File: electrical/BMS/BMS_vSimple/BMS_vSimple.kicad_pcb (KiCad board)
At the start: 2 copper layers, 133.3 x 82.6 mm, 140 parts, among them J1 Conn_01x04_Pin, J2 Conn_02x12_Top_Bottom, J3 Conn_01x13_Socket, Q6 BCP56, U1 STM32F412RGTx, U2 BQ79652PAPRQ1, U3 ISO1044BD, U4 CD74HC4067M

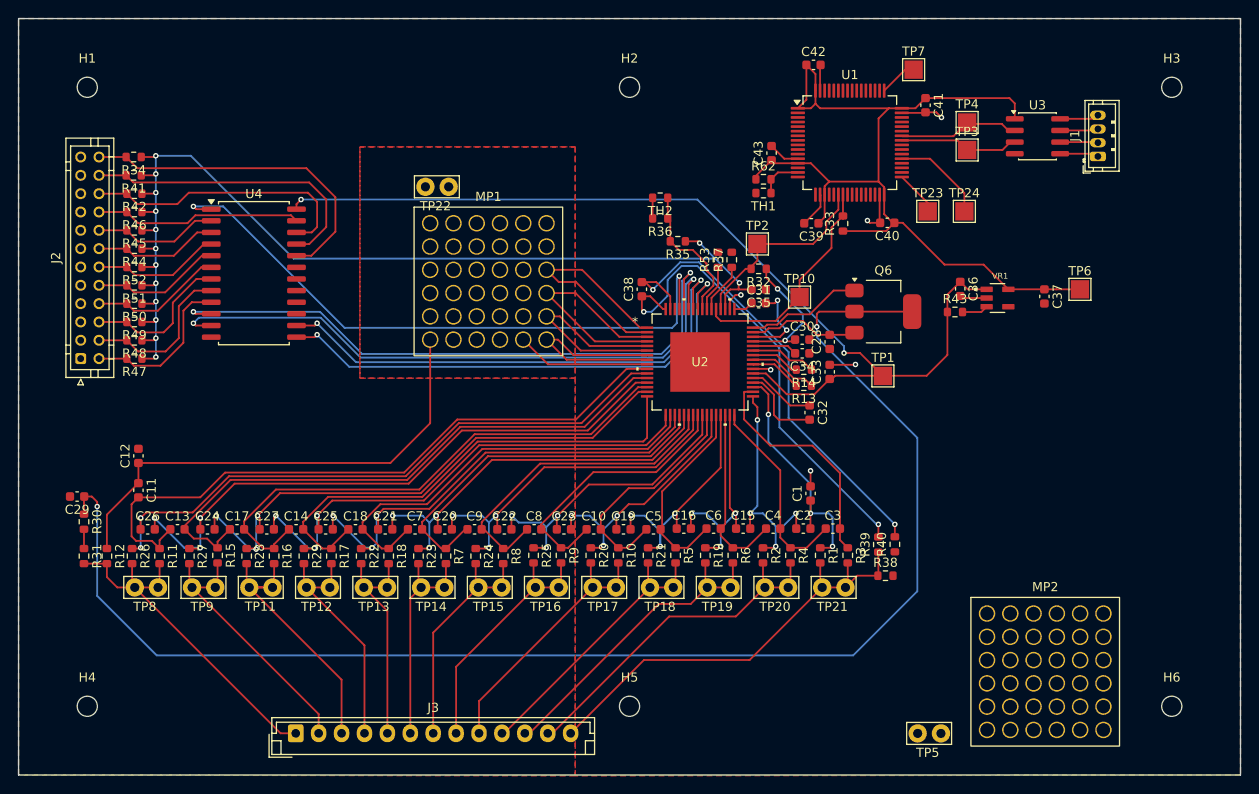
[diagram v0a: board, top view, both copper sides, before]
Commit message: bms is smaller now...
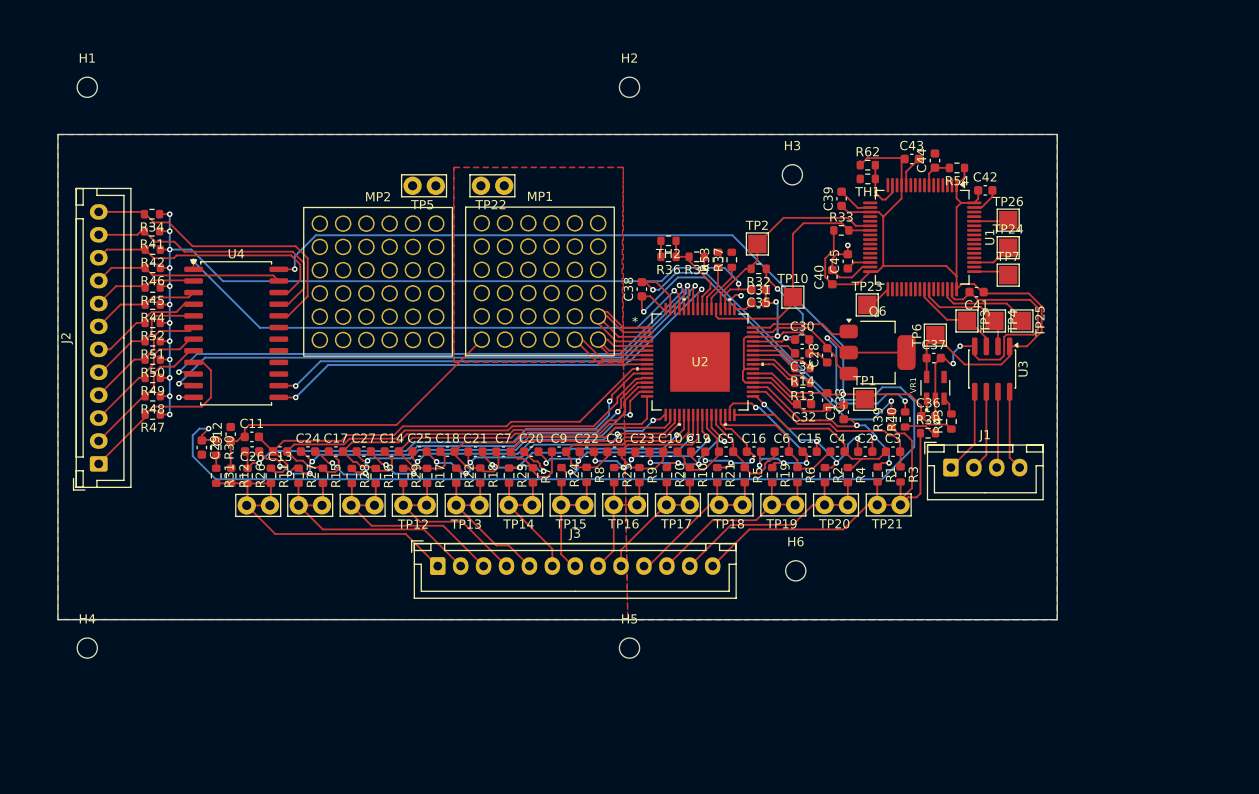
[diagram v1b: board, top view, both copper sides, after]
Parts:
- added C44: 100n, Capacitor_SMD:C_0603_1608Metric, F.Cu at (127.3, 75.8)
- added C45: 4.7u, Capacitor_SMD:C_0603_1608Metric, F.Cu at (117.8, 86.8)
- added R54: 10k, Resistor_SMD:R_0603_1608Metric, F.Cu at (129.7, 76.5)
- added TP25: TestPoint, TestPoint:TestPoint_Pad_2.0x2.0mm, F.Cu at (136.8, 93.2)
- added TP26: TestPoint, TestPoint:TestPoint_Pad_2.0x2.0mm, F.Cu at (135.2, 82.2)
- J1: footprint Connector_JST:JST_ZH_B4B-ZR_1x04_P1.50mm_Vertical -> Connector_JST:JST_XH_B4B-XH-A_1x04_P2.50mm_Vertical
- J2: value Conn_02x12_Top_Bottom -> Conn_01x12; footprint Connector_JST:JST_PHD_B24B-PHDSS_2x12_P2.00mm_Vertical -> Connector_JST:JST_XH_B12B-XH-A_1x12_P2.50mm_Vertical
- J3: footprint Connector_JST:JST_EH_B13B-EH-A_1x13_P2.50mm_Vertical -> Connector_JST:JST_XH_B13B-XH-A_1x13_P2.50mm_Vertical
- moved MP2 84.3 mm to (66.5, 89.0)
- moved TP5 81.3 mm to (70.2, 78.5)
- moved H6 43.6 mm to (112.1, 120.5)
- moved H3 42.5 mm to (111.7, 77.3)
- moved J1 37.6 mm to (129.0, 109.2), turned to 0 degrees
- moved U3 25.9 mm to (133.5, 98.5), turned to -90 degrees
- moved TP7 24.7 mm to (135.2, 88.2)
- moved J3 23.9 mm to (73.0, 120.0)
- moved C42 23.2 mm to (132.8, 79.0)
- moved TP4 21.9 mm to (133.8, 93.2), turned to -90 degrees
- moved C41 21.1 mm to (131.8, 90.1), turned to 180 degrees
- moved TP3 18.7 mm to (130.8, 93.2), turned to -90 degrees
- moved R31 16.9 mm to (48.8, 110.1)
- moved TP6 16.6 mm to (127.3, 94.8), turned to 90 degrees
- moved R30 16.6 mm to (48.8, 107.1)
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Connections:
- J2 pad 1: GND -> Net-(J2-Pin_1)
- J2 pad 11: GND -> Net-(J2-Pin_11)
- J2 pad 3: GND -> Net-(J2-Pin_3)
- J2 pad 5: GND -> Net-(J2-Pin_5)
- J2 pad 7: GND -> Net-(J2-Pin_7)
- J2 pad 9: GND -> Net-(J2-Pin_9)
- R34 pad 2: Net-(J2-Pin_24) -> Net-(J2-Pin_12)
- R41 pad 2: Net-(J2-Pin_22) -> Net-(J2-Pin_11)
- R42 pad 2: Net-(J2-Pin_20) -> Net-(J2-Pin_10)
- R44 pad 2: Net-(J2-Pin_14) -> Net-(J2-Pin_7)
- R45 pad 2: Net-(J2-Pin_16) -> Net-(J2-Pin_8)
- R46 pad 2: Net-(J2-Pin_18) -> Net-(J2-Pin_9)
- R47 pad 2: Net-(J2-Pin_2) -> Net-(J2-Pin_1)
- R48 pad 2: Net-(J2-Pin_4) -> Net-(J2-Pin_2)
- R49 pad 2: Net-(J2-Pin_6) -> Net-(J2-Pin_3)
- R50 pad 2: Net-(J2-Pin_8) -> Net-(J2-Pin_4)
- R51 pad 2: Net-(J2-Pin_10) -> Net-(J2-Pin_5)
- R52 pad 2: Net-(J2-Pin_12) -> Net-(J2-Pin_6)
- TP24 pad 1: Net-(U1-PC6) -> Net-(U1-PC10)
- U1 pad 30: unconnected-(U1-VCAP_1-Pad30) -> Net-(U1-VCAP_1)
- U1 pad 37: Net-(U1-PC6) -> unconnected-(U1-PC6-Pad37)
- U1 pad 46: unconnected-(U1-PA13-Pad46) -> Net-(U1-PA13)
- U1 pad 51: unconnected-(U1-PC10-Pad51) -> Net-(U1-PC10)
- U1 pad 60: unconnected-(U1-BOOT0-Pad60) -> Net-(U1-BOOT0)
- U1 pad 7: unconnected-(U1-NRST-Pad7) -> Net-(U1-NRST)
- U4 pad 2: Net-(J2-Pin_16) -> Net-(J2-Pin_8)
- U4 pad 20: Net-(J2-Pin_24) -> Net-(J2-Pin_12)
- U4 pad 21: Net-(J2-Pin_22) -> Net-(J2-Pin_11)
- U4 pad 22: Net-(J2-Pin_20) -> Net-(J2-Pin_10)
- U4 pad 23: Net-(J2-Pin_18) -> Net-(J2-Pin_9)
- U4 pad 3: Net-(J2-Pin_14) -> Net-(J2-Pin_7)
- U4 pad 4: Net-(J2-Pin_12) -> Net-(J2-Pin_6)
- U4 pad 5: Net-(J2-Pin_10) -> Net-(J2-Pin_5)
- U4 pad 6: Net-(J2-Pin_8) -> Net-(J2-Pin_4)
- U4 pad 7: Net-(J2-Pin_6) -> Net-(J2-Pin_3)
- U4 pad 8: Net-(J2-Pin_4) -> Net-(J2-Pin_2)
- U4 pad 9: Net-(J2-Pin_2) -> Net-(J2-Pin_1)
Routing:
- net /BAT+: track 170.0 -> 96.6 mm
- net GND: track 51.8 -> 102.7 mm, vias 8 -> 7
- net Net-(J2-Pin_24): track 36.7 -> 0.00 mm
- net Net-(C29-Pad1): track 154.3 -> 119.6 mm
- net Net-(J2-Pin_22): track 32.9 -> 0.00 mm
- net Net-(J2-Pin_20): track 30.4 -> 0.00 mm
- net Net-(J2-Pin_11): track 0.00 -> 30.2 mm
- net Net-(J2-Pin_18): track 22.7 -> 0.00 mm
- net Net-(J2-Pin_9): track 0.00 -> 20.8 mm
- net Net-(J2-Pin_1): track 0.00 -> 20.7 mm
- net /CB12: track 72.1 -> 51.5 mm
- net Net-(J2-Pin_12): track 14.0 -> 33.2 mm
- net /VC9: track 56.9 -> 39.5 mm, vias 3 -> 4
- net /VC8: track 51.6 -> 34.5 mm, vias 3 -> 4
- net /VC12: track 67.3 -> 50.9 mm
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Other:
- board size 133.3 x 82.6 mm -> 109 x 52.9 mm
